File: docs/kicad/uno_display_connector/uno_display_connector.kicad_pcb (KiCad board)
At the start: 2 copper layers, 3 parts, among them J1 Conn_01x08, J2 Conn_01x08, U1 uno_display

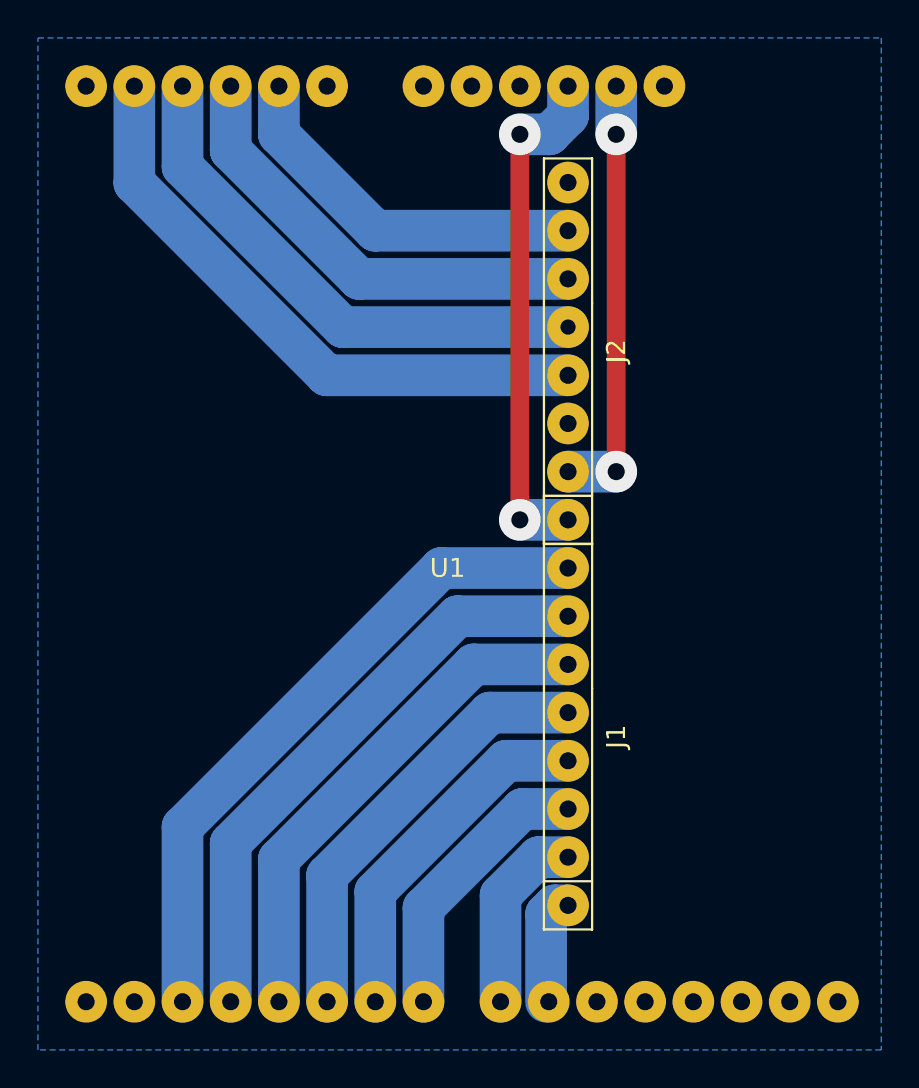
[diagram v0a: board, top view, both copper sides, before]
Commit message: start MAKE NEW motherboard and display_connector FOR olds TeensyExprssion box with TE2 code
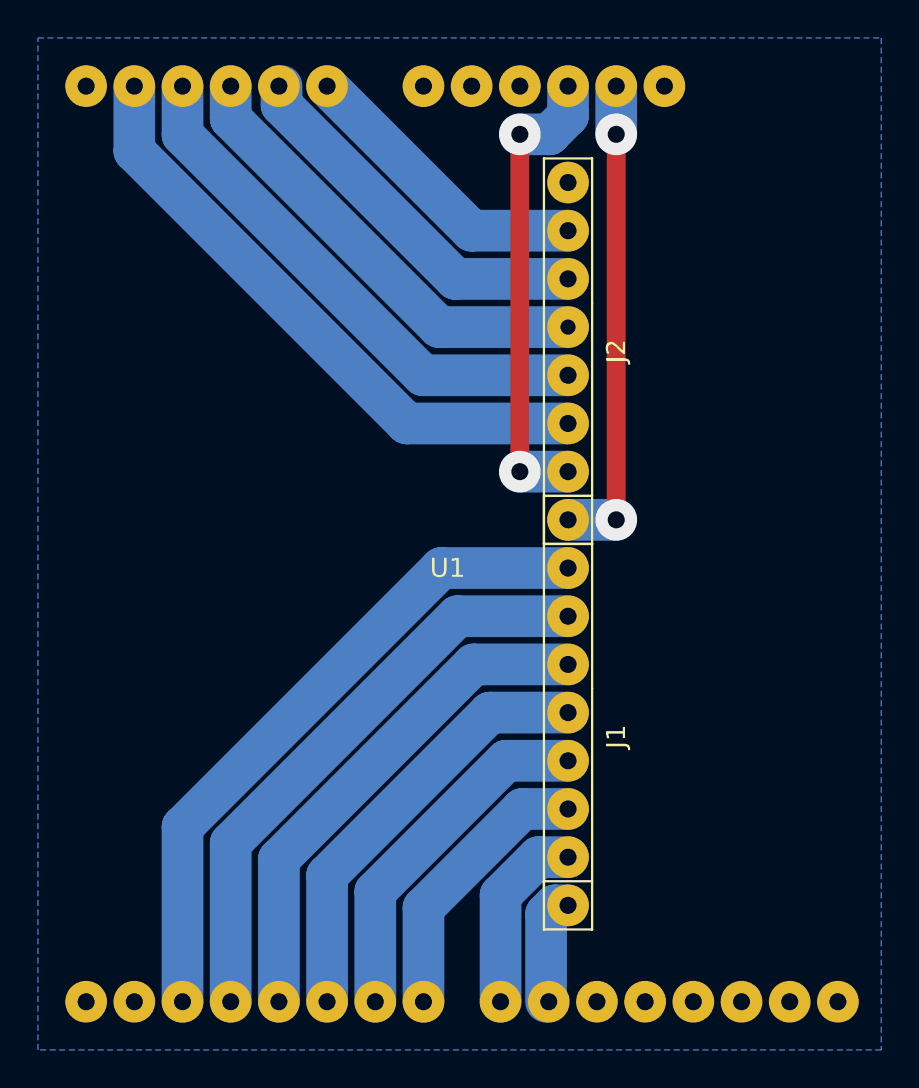
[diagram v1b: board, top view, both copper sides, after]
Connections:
- J2 pad 1: +5V -> +3V3
- J2 pad 2: +3V3 -> +5V
- U1 pad 23: (no net) -> LCD_RD
- U1 pad 24: LCD_RD -> LCD_WR
- U1 pad 25: LCD_WR -> LCD_RS
- U1 pad 26: LCD_RS -> LCD_CS
- U1 pad 27: LCD_CS -> LCD_RST
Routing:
- net LCD_RST: track 0.00 -> 32.2 mm
- net LCD_WR: track 24.0 -> 19.9 mm
- net LCD_RD: track 19.9 -> 15.9 mm
- net LCD_RS: track 28.1 -> 24.0 mm
- net LCD_CS: track 32.2 -> 28.1 mm
- net +5V: track 27.4 -> 24.8 mm
- net +3V3: track 22.9 -> 25.4 mm
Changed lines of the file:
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@@
   )
   (setup
-    (last_trace_width 2.2)
+    (last_trace_width 1)
     (user_trace_width 1)
     (user_trace_width 2)
@@
     (pad_to_mask_clearance 0.05)
     (aux_axis_origin 0 0)
-    (visible_elements FFFFFF7F)
+    (visible_elements 7FFFFFFF)
     (pcbplotparams
       (layerselection 0x010fc_ffffffff)
@@
       (effects (font (size 1 1) (thickness 0.15)))
     )
+    (fp_line (start -6.35 -1.27) (end -6.35 1.27) (layer F.SilkS) (width 0.12))
+    (fp_line (start -8.89 -1.27) (end -6.35 -1.27) (layer F.SilkS) (width 0.12))
+    (fp_line (start 3.81 -1.27) (end -8.89 -1.27) (layer F.SilkS) (width 0.12))
+    (fp_line (start -8.89 1.27) (end 3.81 1.27) (layer F.SilkS) (width 0.12))
+    (fp_line (start -8.89 -1.27) (end -8.89 1.27) (layer F.SilkS) (width 0.12))
+    (fp_line (start 3.81 -1.27) (end 11.43 -1.27) (layer F.SilkS) (width 0.12))
+    (fp_line (start 11.43 -1.27) (end 11.43 1.27) (layer F.SilkS) (width 0.12))
     (fp_line (start 11.43 1.27) (end 3.81 1.27) (layer F.SilkS) (width 0.12))
-    (fp_line (start 11.43 -1.27) (end 11.43 1.27) (layer F.SilkS) (width 0.12))
-    (fp_line (start 3.81 -1.27) (end 11.43 -1.27) (layer F.SilkS) (width 0.12))
-    (fp_line (start -8.89 -1.27) (end -8.89 1.27) (layer F.SilkS) (width 0.12))
-    (fp_line (start -8.89 1.27) (end 3.81 1.27) (layer F.SilkS) (width 0.12))
-    (fp_line (start 3.81 -1.27) (end -8.89 -1.27) (layer F.SilkS) (width 0.12))
-    (fp_line (start -8.89 -1.27) (end -6.35 -1.27) (layer F.SilkS) (width 0.12))
-    (fp_line (start -6.35 -1.27) (end -6.35 1.27) (layer F.SilkS) (width 0.12))
     (pad 1 thru_hole circle (at -7.62 0 90) (size 2.2 2.2) (drill 0.9) (layers *.Cu *.Mask)
       (net 1 LCD_D1))
@@
       (effects (font (size 1 1) (thickness 0.15)))
     )
+    (fp_line (start 11.43 1.27) (end 3.81 1.27) (layer F.SilkS) (width 0.12))
+    (fp_line (start 11.43 -1.27) (end 11.43 1.27) (layer F.SilkS) (width 0.12))
+    (fp_line (start 3.81 -1.27) (end 11.43 -1.27) (layer F.SilkS) (width 0.12))
+    (fp_line (start -8.89 -1.27) (end -8.89 1.27) (layer F.SilkS) (width 0.12))
+    (fp_line (start -8.89 1.27) (end 3.81 1.27) (layer F.SilkS) (width 0.12))
+    (fp_line (start 3.81 -1.27) (end -8.89 -1.27) (layer F.SilkS) (width 0.12))
+    (fp_line (start -8.89 -1.27) (end -6.35 -1.27) (layer F.SilkS) (width 0.12))
     (fp_line (start -6.35 -1.27) (end -6.35 1.27) (layer F.SilkS) (width 0.12))
-    (fp_line (start -8.89 -1.27) (end -6.35 -1.27) (layer F.SilkS) (width 0.12))
-    (fp_line (start 3.81 -1.27) (end -8.89 -1.27) (layer F.SilkS) (width 0.12))
-    (fp_line (start -8.89 1.27) (end 3.81 1.27) (layer F.SilkS) (width 0.12))
-    (fp_line (start -8.89 -1.27) (end -8.89 1.27) (layer F.SilkS) (width 0.12))
-    (fp_line (start 3.81 -1.27) (end 11.43 -1.27) (layer F.SilkS) (width 0.12))
-    (fp_line (start 11.43 -1.27) (end 11.43 1.27) (layer F.SilkS) (width 0.12))
-    (fp_line (start 11.43 1.27) (end 3.81 1.27) (layer F.SilkS) (width 0.12))
     (pad 8 thru_hole circle (at 10.16 0 90) (size 2.2 2.2) (drill 0.9) (layers *.Cu *.Mask)
       (net 9 GND))
@@
       (net 15 LCD_RST))
     (pad 2 thru_hole circle (at -5.08 0 90) (size 2.2 2.2) (drill 0.9) (layers *.Cu *.Mask)
+      (net 16 +5V))
+    (pad 1 thru_hole circle (at -7.62 0 90) (size 2.2 2.2) (drill 0.9) (layers *.Cu *.Mask)
       (net 10 +3V3))
-    (pad 1 thru_hole circle (at -7.62 0 90) (size 2.2 2.2) (drill 0.9) (layers *.Cu *.Mask)
-      (net 16 +5V))
   )
   (module 0_my_footprints:unoDisplay (layer F.Cu)
@@
       (effects (font (size 1 1) (thickness 0.15)))
     )
+    (fp_line (start -22.86 -27.94) (end -22.86 25.4) (layer F.Fab) (width 0.12))
+    (fp_line (start -22.86 -27.94) (end 21.59 -27.94) (layer F.Fab) (width 0.12))
+    (fp_line (start 21.59 -27.94) (end 21.59 25.4) (layer F.Fab) (width 0.12))
     (fp_line (start -22.86 25.4) (end 21.59 25.4) (layer F.Fab) (width 0.12))
-    (fp_line (start 21.59 -27.94) (end 21.59 25.4) (layer F.Fab) (width 0.12))
-    (fp_line (start -22.86 -27.94) (end 21.59 -27.94) (layer F.Fab) (width 0.12))
-    (fp_line (start -22.86 -27.94) (end -22.86 25.4) (layer F.Fab) (width 0.12))
     (pad 1 thru_hole circle (at 19.05 -25.4) (size 2.2 2.2) (drill 0.9) (layers *.Cu *.Mask)
       (net 17 "Net-(U1-Pad1)"))
@@
     (pad 22 thru_hole circle (at 1.27 22.86) (size 2.2 2.2) (drill 0.9) (layers *.Cu *.Mask)
       (net 27 "Net-(U1-Pad22)"))
-    (pad 23 thru_hole circle (at 6.35 22.86) (size 2.2 2.2) (drill 0.9) (layers *.Cu *.Mask))
+    (pad 23 thru_hole circle (at 6.35 22.86) (size 2.2 2.2) (drill 0.9) (layers *.Cu *.Mask)
+      (net 11 LCD_RD))
     (pad 24 thru_hole circle (at 8.89 22.86) (size 2.2 2.2) (drill 0.9) (layers *.Cu *.Mask)
-      (net 11 LCD_RD))
+      (net 12 LCD_WR))
     (pad 25 thru_hole circle (at 11.43 22.86) (size 2.2 2.2) (drill 0.9) (layers *.Cu *.Mask)
-      (net 12 LCD_WR))
+      (net 13 LCD_RS))
     (pad 26 thru_hole circle (at 13.97 22.86) (size 2.2 2.2) (drill 0.9) (layers *.Cu *.Mask)
-      (net 13 LCD_RS))
+      (net 14 LCD_CS))
     (pad 27 thru_hole circle (at 16.51 22.86) (size 2.2 2.2) (drill 0.9) (layers *.Cu *.Mask)
-      (net 14 LCD_CS))
+      (net 15 LCD_RST))
     (pad 28 thru_hole circle (at 19.05 22.86) (size 2.2 2.2) (drill 0.9) (layers *.Cu *.Mask)
       (net 28 "Net-(U1-Pad28)"))
@@
   (segment (start 21.25961 -25.4) (end 27.94 -25.4) (width 2.2) (layer B.Cu) (net 8))
   (segment (start 30.48 -50.8) (end 30.48 -48.26) (width 2.2) (layer B.Cu) (net 10))
-  (segment (start 27.94 -30.48) (end 30.48 -30.48) (width 2.2) (layer B.Cu) (net 10))
-  (segment (start 30.48 -30.48) (end 30.48 -30.48) (width 2.2) (layer B.Cu) (net 10))
-  (via (at 30.48 -30.48) (size 2.2) (drill 0.9) (layers F.Cu B.Cu) (net 10))
+  (segment (start 27.94 -27.94) (end 30.48 -27.94) (width 2.2) (layer B.Cu) (net 10))
+  (via (at 30.48 -27.94) (size 2.2) (drill 0.9) (layers F.Cu B.Cu) (net 10))
   (segment (start 30.48 -48.26) (end 30.48 -48.26) (width 2.2) (layer B.Cu) (net 10))
   (via (at 30.48 -48.26) (size 2.2) (drill 0.9) (layers F.Cu B.Cu) (net 10))
-  (segment (start 30.48 -48.26) (end 30.48 -30.48) (width 1) (layer F.Cu) (net 10))
-  (segment (start 12.7 -48.26) (end 12.7 -50.8) (width 2.2) (layer B.Cu) (net 11))
-  (segment (start 17.78 -43.18) (end 12.7 -48.26) (width 2.2) (layer B.Cu) (net 11))
-  (segment (start 27.94 -43.18) (end 17.78 -43.18) (width 2.2) (layer B.Cu) (net 11))
-  (segment (start 10.16 -47.405874) (end 10.16 -50.8) (width 2.2) (layer B.Cu) (net 12))
-  (segment (start 16.925874 -40.64) (end 10.16 -47.405874) (width 2.2) (layer B.Cu) (net 12))
-  (segment (start 27.94 -40.64) (end 16.925874 -40.64) (width 2.2) (layer B.Cu) (net 12))
-  (segment (start 7.62 -46.551748) (end 7.62 -50.8) (width 2.2) (layer B.Cu) (net 13))
-  (segment (start 16.071748 -38.1) (end 7.62 -46.551748) (width 2.2) (layer B.Cu) (net 13))
-  (segment (start 27.94 -38.1) (end 16.071748 -38.1) (width 2.2) (layer B.Cu) (net 13))
-  (segment (start 5.08 -45.697622) (end 5.08 -50.8) (width 2.2) (layer B.Cu) (net 14))
-  (segment (start 15.217622 -35.56) (end 5.08 -45.697622) (width 2.2) (layer B.Cu) (net 14))
-  (segment (start 27.94 -35.56) (end 15.217622 -35.56) (width 2.2) (layer B.Cu) (net 14))
-  (segment (start 27.94 -27.94) (end 25.4 -27.94) (width 2.2) (layer B.Cu) (net 16))
+  (segment (start 30.48 -48.26) (end 30.48 -27.94) (width 1) (layer F.Cu) (net 10))
+  (segment (start 27.94 -43.18) (end 22.86 -43.18) (width 2.2) (layer B.Cu) (net 11))
+  (segment (start 22.86 -43.18) (end 15.24 -50.8) (width 2.2) (layer B.Cu) (net 11))
+  (segment (start 22.005874 -40.64) (end 12.839991 -49.805883) (width 2.2) (layer B.Cu) (net 12))
+  (segment (start 27.94 -40.64) (end 22.005874 -40.64) (width 2.2) (layer B.Cu) (net 12))
+  (segment (start 12.839991 -49.805883) (end 12.839991 -50.8) (width 2.2) (layer B.Cu) (net 12))
+  (segment (start 21.151748 -38.1) (end 10.16 -49.091748) (width 2.2) (layer B.Cu) (net 13))
+  (segment (start 27.94 -38.1) (end 21.151748 -38.1) (width 2.2) (layer B.Cu) (net 13))
+  (segment (start 10.16 -49.091748) (end 10.16 -50.8) (width 2.2) (layer B.Cu) (net 13))
+  (segment (start 20.297622 -35.56) (end 7.62 -48.237622) (width 2.2) (layer B.Cu) (net 14))
+  (segment (start 27.94 -35.56) (end 20.297622 -35.56) (width 2.2) (layer B.Cu) (net 14))
+  (segment (start 7.62 -48.237622) (end 7.62 -50.8) (width 2.2) (layer B.Cu) (net 14))
+  (segment (start 19.443496 -33.02) (end 5.08 -47.383496) (width 2.2) (layer B.Cu) (net 15))
+  (segment (start 27.94 -33.02) (end 19.443496 -33.02) (width 2.2) (layer B.Cu) (net 15))
+  (segment (start 5.08 -47.383496) (end 5.08 -50.8) (width 2.2) (layer B.Cu) (net 15))
+  (segment (start 27.94 -30.48) (end 25.4 -30.48) (width 2.2) (layer B.Cu) (net 16))
   (segment (start 27.94 -49.244366) (end 26.955634 -48.26) (width 2.2) (layer B.Cu) (net 16))
   (segment (start 27.94 -50.8) (end 27.94 -49.244366) (width 2.2) (layer B.Cu) (net 16))
   (segment (start 26.955634 -48.26) (end 25.4 -48.26) (width 2.2) (layer B.Cu) (net 16))
-  (segment (start 25.4 -27.94) (end 25.4 -27.94) (width 2.2) (layer B.Cu) (net 16))
-  (via (at 25.4 -27.94) (size 2.2) (drill 0.9) (layers F.Cu B.Cu) (net 16))
+  (via (at 25.4 -30.48) (size 2.2) (drill 0.9) (layers F.Cu B.Cu) (net 16))
   (segment (start 25.4 -48.26) (end 25.4 -48.26) (width 2.2) (layer B.Cu) (net 16))
   (via (at 25.4 -48.26) (size 2.2) (drill 0.9) (layers F.Cu B.Cu) (net 16))
-  (segment (start 25.4 -48.26) (end 25.4 -27.94) (width 1) (layer F.Cu) (net 16))
+  (segment (start 25.4 -48.26) (end 25.4 -30.48) (width 1) (layer F.Cu) (net 16))
   (zone (net 9) (net_name GND) (layer B.Cu) (hatch edge 0.508)
     (connect_pads yes (clearance 0.3))
